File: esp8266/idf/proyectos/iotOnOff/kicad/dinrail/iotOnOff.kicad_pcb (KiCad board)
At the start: 2 copper layers, 82 x 32 mm, 18 parts, among them J1 Conn_01x02, J2 Conn_01x02, J3 Conn_01x04, K1 SANYOU_SRD_Form_A, Q1 2N7002, SW1 SW_Push, U1 AMS1117-3.3, U3 ESP-12F

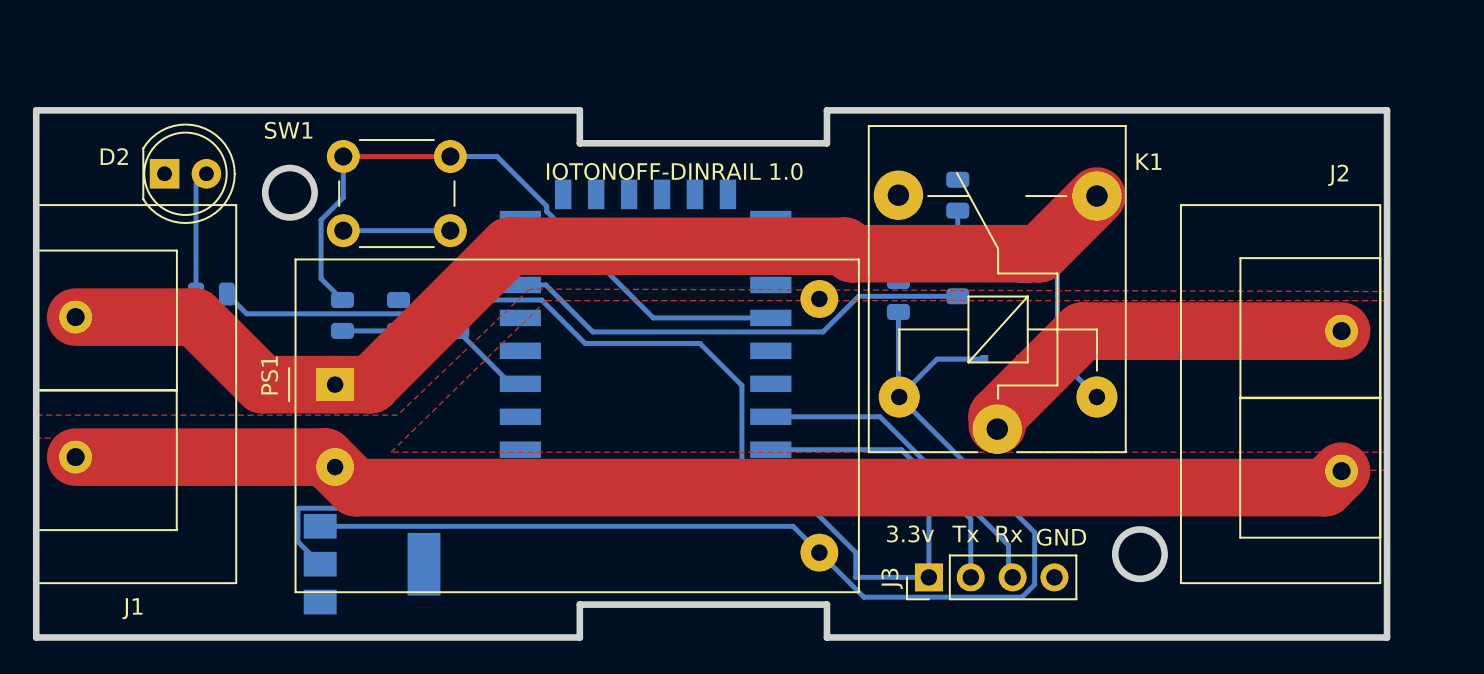
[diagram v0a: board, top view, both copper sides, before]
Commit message: ff
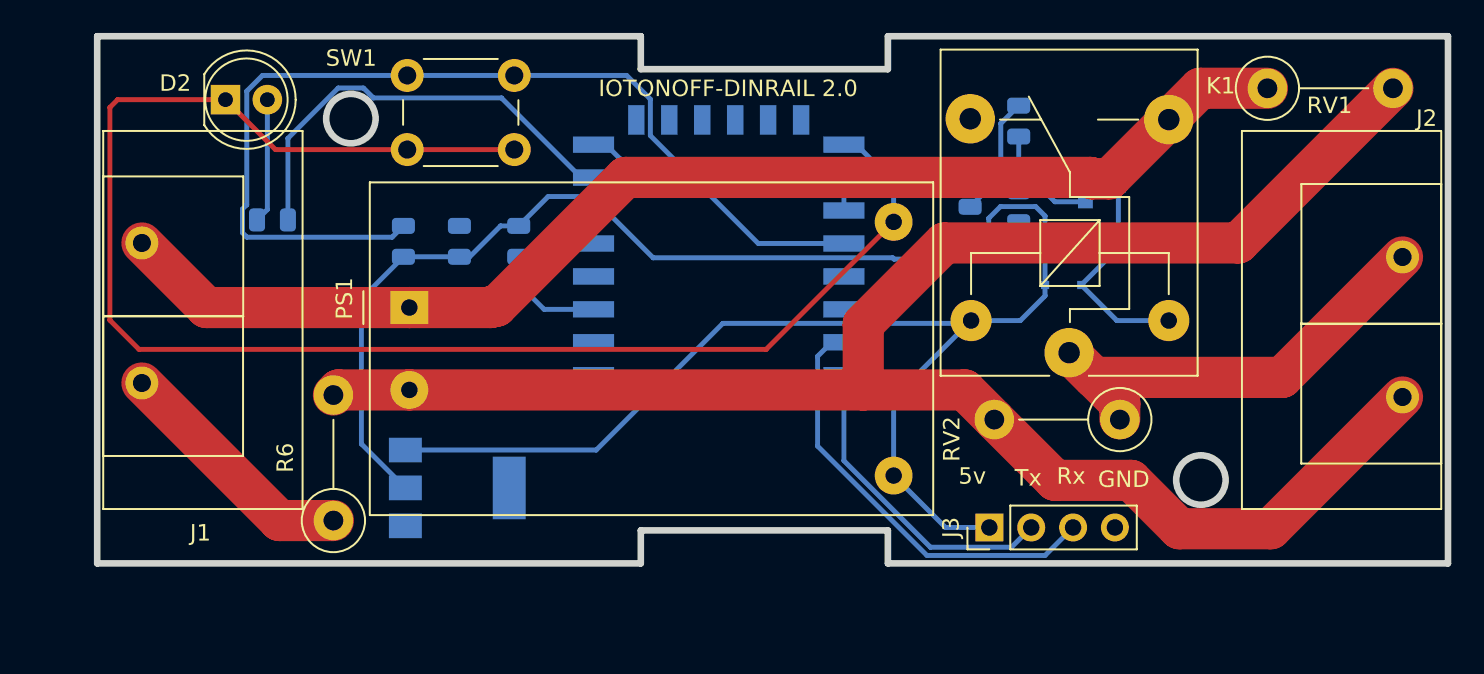
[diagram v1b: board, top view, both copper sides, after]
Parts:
- added R6: 10, Resistor_THT:R_Axial_DIN0411_L9.9mm_D3.6mm_P7.62mm_Vertical, F.Cu at (117.2, 104.0)
- added RV1: Varistor, Resistor_THT:R_Axial_DIN0411_L9.9mm_D3.6mm_P7.62mm_Vertical, F.Cu at (173.9, 77.7)
- added RV2: Varistor, Resistor_THT:R_Axial_DIN0411_L9.9mm_D3.6mm_P7.62mm_Vertical, F.Cu at (164.9, 97.8)
- moved U1 6.94 mm to (124.7, 102.0)
- moved PS1 6.50 mm to (121.8, 91.0)
- moved K1 6.37 mm to (161.9, 93.8)
- moved U3 6.34 mm to (140.6, 91.6)
- moved C1 6.27 mm to (155.8, 85.8)
- moved SW1 6.27 mm to (121.7, 76.9)
- moved J1 6.04 mm to (103.2, 103.2)
- moved R2 5.83 mm to (158.8, 84.9)
- moved R3 5.83 mm to (158.8, 79.7)
- moved D2 5.83 mm to (110.7, 78.4)
- moved R1 5.83 mm to (121.5, 87.0)
- moved R4 5.83 mm to (113.5, 85.7)
- moved C2 5.83 mm to (124.8, 87.0)
- moved D1 5.83 mm to (161.5, 89.7)
- moved J2 5.83 mm to (184.4, 80.3)
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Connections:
- J2 pad 2: Net-(J1-Pad1) -> Net-(J2-Pad2)
- J3 pad 1: Net-(C2-Pad1) -> Net-(C1-Pad1)
- PS1 pad 2: Net-(J1-Pad1) -> Net-(J2-Pad2)
- U3 pad 1: Net-(U3-Pad1) -> unconnected-(U3-Pad1)
- U3 pad 10: Net-(U3-Pad10) -> unconnected-(U3-Pad10)
- U3 pad 11: Net-(U3-Pad11) -> unconnected-(U3-Pad11)
- U3 pad 12: Net-(U3-Pad12) -> unconnected-(U3-Pad12)
- U3 pad 13: Net-(U3-Pad13) -> unconnected-(U3-Pad13)
- U3 pad 14: Net-(U3-Pad14) -> unconnected-(U3-Pad14)
- U3 pad 17: Net-(U3-Pad17) -> Net-(U3-Pad16)
- U3 pad 19: Net-(U3-Pad19) -> unconnected-(U3-Pad19)
- U3 pad 2: Net-(U3-Pad2) -> unconnected-(U3-Pad2)
- U3 pad 20: Net-(U3-Pad20) -> unconnected-(U3-Pad20)
- U3 pad 4: Net-(U3-Pad4) -> unconnected-(U3-Pad4)
- U3 pad 5: Net-(U3-Pad5) -> unconnected-(U3-Pad5)
- U3 pad 9: Net-(U3-Pad9) -> unconnected-(U3-Pad9)
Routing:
- net Net-(J2-Pad2): track 0.00 -> 113.9 mm
- net GND: track 6.50 -> 104.2 mm
- net Net-(C2-Pad1): track 104.7 -> 34.9 mm
- net Net-(J1-Pad1): track 78.0 -> 15.1 mm
- net Net-(R1-Pad1): track 40.0 -> 61.0 mm
- net Net-(R4-Pad2): track 19.9 -> 27.0 mm
- net Net-(J1-Pad2): track 68.8 -> 75.5 mm
- net Net-(J3-Pad3): track 19.7 -> 26.4 mm
- net Net-(J2-Pad1): track 23.6 -> 29.2 mm
- net Net-(U3-Pad16): track 0.00 -> 2.00 mm
- net Net-(J3-Pad2): track 17.4 -> 19.2 mm
- net Net-(D1-Pad2): track 14.9 -> 13.1 mm
- net Net-(R5-Pad1): track 5.13 -> 6.83 mm
- net Net-(R2-Pad2): track 28.6 -> 28.0 mm
- removed copper zone on F.Cu, net Net-(J1-Pad1)
- removed copper zone on F.Cu, net Net-(J1-Pad2)
- removed copper zone on F.Cu, net Net-(J2-Pad1)
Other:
- net class AC removed
- net class Default removed
- board text added: "5v"
- board text added: "IOTONOFF-DINRAIL 2.0"
- board text removed: "3.3v"
- board text removed: "IOTONOFF-DINRAIL 1.0"
